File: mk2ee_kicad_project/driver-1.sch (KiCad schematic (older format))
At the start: 37 parts, among them J3 Conn_01x02_Male, J4 Conn_02x03_Male, J5 Conn_02x03_Male, J6 Conn_01x04_Male, J7 Conn_01x04_Male, U4 TSR_1-2465, U5 NCP718xSN330, U6 74HC595, U7 DRV8818PWP

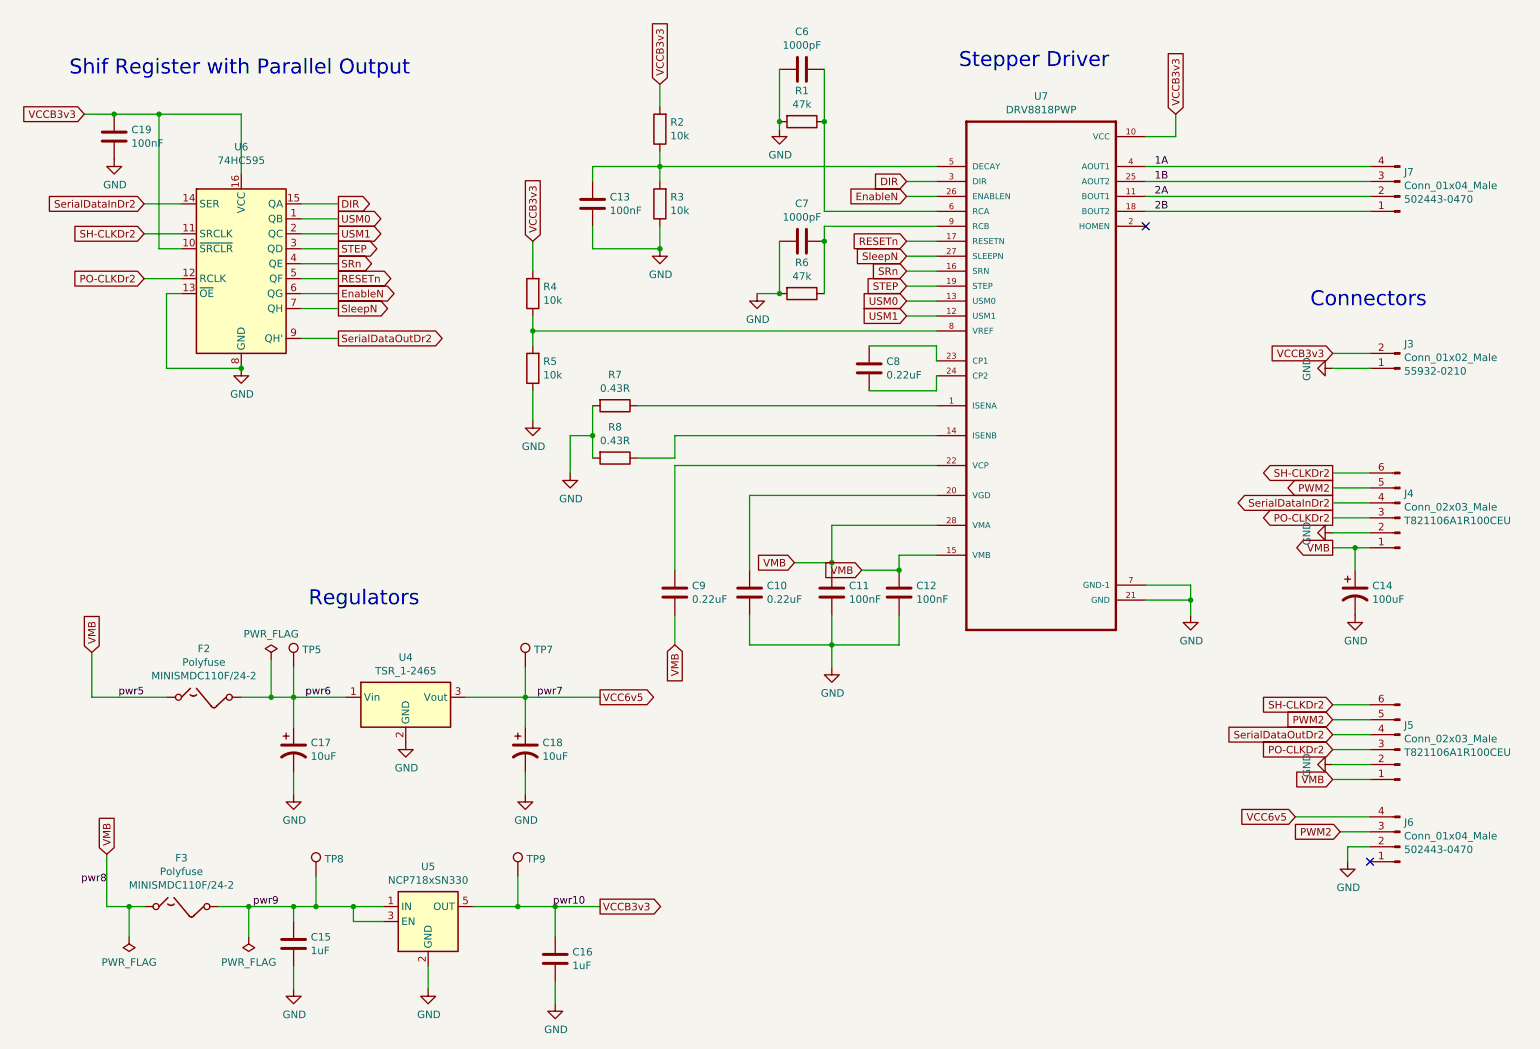
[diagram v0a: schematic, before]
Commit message: all components are connected
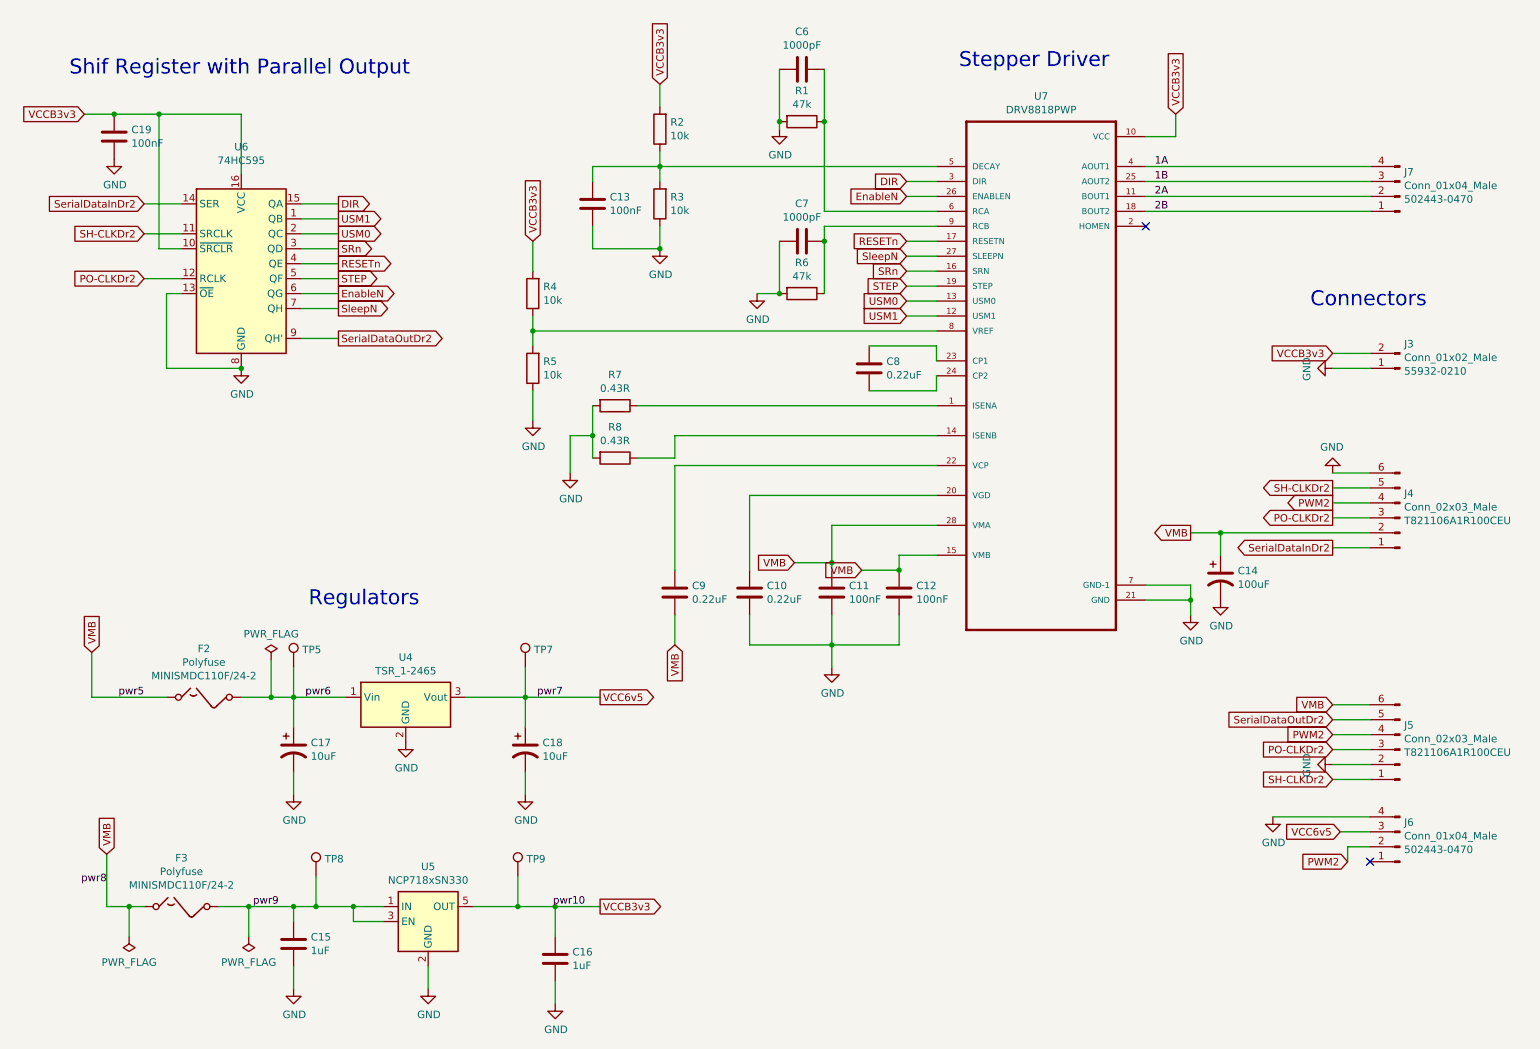
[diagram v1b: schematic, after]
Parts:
- TP5, TP7, TP8, TP9: footprint TestPoint:TestPoint_Pad_D4.0mm -> TestPoint:TestPoint_Pad_D1.5mm
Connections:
- net GND: now also J4.6 (Pin_6), J6.4 (Pin_4); no longer J4.2 (Pin_2), J6.2 (Pin_2)
- net PWM2: now also J4.4 (Pin_4), J5.4 (Pin_4), J6.2 (Pin_2); no longer J4.5 (Pin_5), J5.5 (Pin_5), J6.3 (Pin_3)
- net RESETn: now also U6.4 (QE); no longer U6.5 (QF)
- net SH-CLKDr2: now also J4.5 (Pin_5), J5.1 (Pin_1); no longer J4.6 (Pin_6), J5.6 (Pin_6)
- net SRn: now also U6.3 (QD); no longer U6.4 (QE)
- net STEP: now also U6.5 (QF); no longer U6.3 (QD)
- net SerialDataInDr2: now also J4.1 (Pin_1); no longer J4.4 (Pin_4)
- net SerialDataOutDr2: now also J5.5 (Pin_5); no longer J5.4 (Pin_4)
- net USM0: now also U6.2 (QC); no longer U6.1 (QB)
- net USM1: now also U6.1 (QB); no longer U6.2 (QC)
- net VCC6v5: now also J6.3 (Pin_3); no longer J6.4 (Pin_4)
- net VMB: now also J4.2 (Pin_2), J5.6 (Pin_6); no longer J4.1 (Pin_1), J5.1 (Pin_1)
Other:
- moved on the sheet: C14
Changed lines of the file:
@@
 L power:GND #PWR0117
 U 1 1 5F4EE14D
-P 9250 4050
-F 0 "#PWR0117" H 9250 3800 50  0001 C CNN
-F 1 "GND" H 9255 3877 50  0000 C CNN
-F 2 "" H 9250 4050 50  0001 C CNN
-F 3 "" H 9250 4050 50  0001 C CNN
-	1    9250 4050
-	0    1    1    0
-$EndComp
-Wire Wire Line
-	9250 4150 9400 4150
-Wire Wire Line
-	9250 4050 9500 4050
+P 9250 3650
+F 0 "#PWR0117" H 9250 3400 50  0001 C CNN
+F 1 "GND" H 9255 3477 50  0000 C CNN
+F 2 "" H 9250 3650 50  0001 C CNN
+F 3 "" H 9250 3650 50  0001 C CNN
+	1    9250 3650
+	-1   0    0    1
+$EndComp
 Text GLabel 2600 1850 2    50   Output ~ 0
 DIR
+Text GLabel 2600 2050 2    50   Output ~ 0
+USM0
 Text GLabel 2600 1950 2    50   Output ~ 0
-USM0
-Text GLabel 2600 2050 2    50   Output ~ 0
 USM1
+Text GLabel 2600 2350 2    50   Output ~ 0
+STEP
 Text GLabel 2600 2150 2    50   Output ~ 0
-STEP
+SRn
 Text GLabel 2600 2250 2    50   Output ~ 0
-SRn
-Text GLabel 2600 2350 2    50   Output ~ 0
 RESETn
+Text GLabel 9250 5300 0    50   Input ~ 0
+SerialDataOutDr2
 Text GLabel 9250 5400 0    50   Input ~ 0
-SerialDataOutDr2
-Text GLabel 9250 5300 0    50   Input ~ 0
 PWM2
-Text GLabel 9250 5200 0    50   Input ~ 0
+Text GLabel 9250 5700 0    50   Input ~ 0
 SH-CLKDr2
 Text GLabel 9250 5500 0    50   Input ~ 0
@@
 Text GLabel 1300 1850 0    50   Input ~ 0
 SerialDataInDr2
-Text GLabel 9250 5700 0    50   Input ~ 0
+Text GLabel 9250 5200 0    50   Input ~ 0
 VMB
 $Comp
@@
 Text GLabel 9250 3950 0    50   Output ~ 0
 PO-CLKDr2
-Text GLabel 9250 3650 0    50   Output ~ 0
+Text GLabel 9250 3750 0    50   Output ~ 0
 SH-CLKDr2
-Text GLabel 9250 3750 0    50   Output ~ 0
+Text GLabel 9250 3850 0    50   Output ~ 0
 PWM2
-Text GLabel 9250 3850 0    50   Output ~ 0
+Text GLabel 9250 4150 0    50   Output ~ 0
 SerialDataInDr2
 $Comp
@@
 Wire Wire Line
 	9250 2950 9500 2950
-Text GLabel 9250 4150 0    50   Output ~ 0
+Text GLabel 8300 4050 0    50   Output ~ 0
 VMB
-Wire Wire Line
-	9400 4300 9400 4150
-Connection ~ 9400 4150
-Wire Wire Line
-	9400 4150 9500 4150
 $Comp
 L power:GND #PWR0137
 U 1 1 5F975427
-P 9400 4600
-F 0 "#PWR0137" H 9400 4350 50  0001 C CNN
-F 1 "GND" H 9405 4427 50  0000 C CNN
-F 2 "" H 9400 4600 50  0001 C CNN
-F 3 "" H 9400 4600 50  0001 C CNN
-	1    9400 4600
+P 8500 4500
+F 0 "#PWR0137" H 8500 4250 50  0001 C CNN
+F 1 "GND" H 8505 4327 50  0000 C CNN
+F 2 "" H 8500 4500 50  0001 C CNN
+F 3 "" H 8500 4500 50  0001 C CNN
+	1    8500 4500
 	1    0    0    -1
 $EndComp
@@
 L power:GND #PWR0145
 U 1 1 5FC7793A
-P 9350 6250
-F 0 "#PWR0145" H 9350 6000 50  0001 C CNN
-F 1 "GND" H 9355 6077 50  0000 C CNN
-F 2 "" H 9350 6250 50  0001 C CNN
-F 3 "" H 9350 6250 50  0001 C CNN
-	1    9350 6250
-	1    0    0    -1
-$EndComp
-Text GLabel 9000 5950 0    50   Input ~ 0
+P 8850 5950
+F 0 "#PWR0145" H 8850 5700 50  0001 C CNN
+F 1 "GND" H 8855 5777 50  0000 C CNN
+F 2 "" H 8850 5950 50  0001 C CNN
+F 3 "" H 8850 5950 50  0001 C CNN
+	1    8850 5950
+	1    0    0    -1
+$EndComp
+Text GLabel 9300 6050 0    50   Input ~ 0
 VCC6v5
 Wire Wire Line
-	9000 5950 9500 5950
-Wire Wire Line
 	9350 6250 9350 6150
 Wire Wire Line
 	9350 6150 9500 6150
-Text GLabel 9300 6050 0    50   Input ~ 0
+Text GLabel 9350 6250 0    50   Input ~ 0
 PWM2
 Wire Wire Line
@@
 L Device:CP1 C?
 U 1 1 602E4B0B
-P 9400 4450
+P 8500 4350
 AR Path="/5F455032/602E4B0B" Ref="C?"  Part="1"
 AR Path="/5F4C637B/602E4B0B" Ref="C?"  Part="1"
 AR Path="/5F475AB3/602E4B0B" Ref="C14"  Part="1"
-F 0 "C14" H 9515 4496 50  0000 L CNN
-F 1 "100uF" H 9515 4405 50  0000 L CNN
-F 2 "Capacitor_SMD:CP_Elec_6.3x7.7" H 9400 4450 50  0001 C CNN
-F 3 "~" H 9400 4450 50  0001 C CNN
-F 4 "EEEFK1E101XP" H 9400 4450 50  0001 C CNN "Name"
-F 5 "Panasonic" H 9400 4450 50  0001 C CNN "Manufacturer"
-	1    9400 4450
+F 0 "C14" H 8615 4396 50  0000 L CNN
+F 1 "100uF" H 8615 4305 50  0000 L CNN
+F 2 "Capacitor_SMD:CP_Elec_6.3x7.7" H 8500 4350 50  0001 C CNN
+F 3 "~" H 8500 4350 50  0001 C CNN
+F 4 "EEEFK1E101XP" H 8500 4350 50  0001 C CNN "Name"
+F 5 "Panasonic" H 8500 4350 50  0001 C CNN "Manufacturer"
+	1    8500 4350
 	1    0    0    -1
 $EndComp
@@
 F 0 "TP5" H 2358 5068 50  0000 L CNN
 F 1 "TestPoint" H 2358 4977 50  0001 L CNN
-F 2 "TestPoint:TestPoint_Pad_D4.0mm" H 2500 4950 50  0001 C CNN
+F 2 "TestPoint:TestPoint_Pad_D1.5mm" H 2500 4950 50  0001 C CNN
 F 3 "~" H 2500 4950 50  0001 C CNN
 	1    2300 4950
@@
 F 0 "TP7" H 3908 5068 50  0000 L CNN
 F 1 "TestPoint" H 3908 4977 50  0001 L CNN
-F 2 "TestPoint:TestPoint_Pad_D4.0mm" H 4050 4950 50  0001 C CNN
+F 2 "TestPoint:TestPoint_Pad_D1.5mm" H 4050 4950 50  0001 C CNN
 F 3 "~" H 4050 4950 50  0001 C CNN
 	1    3850 4950
@@
 F 0 "TP8" H 2508 6468 50  0000 L CNN
 F 1 "TestPoint" H 2508 6377 50  0001 L CNN
-F 2 "TestPoint:TestPoint_Pad_D4.0mm" H 2650 6350 50  0001 C CNN
+F 2 "TestPoint:TestPoint_Pad_D1.5mm" H 2650 6350 50  0001 C CNN
 F 3 "~" H 2650 6350 50  0001 C CNN
 	1    2450 6350
@@
 F 0 "TP9" H 3858 6468 50  0000 L CNN
 F 1 "TestPoint" H 3858 6377 50  0001 L CNN
-F 2 "TestPoint:TestPoint_Pad_D4.0mm" H 4000 6350 50  0001 C CNN
+F 2 "TestPoint:TestPoint_Pad_D1.5mm" H 4000 6350 50  0001 C CNN
 F 3 "~" H 4000 6350 50  0001 C CNN
 	1    3800 6350
@@
 Wire Wire Line
 	5850 2100 5850 2450
+Wire Wire Line
+	8850 5950 9500 5950
+Wire Wire Line
+	9250 4150 9500 4150
+Wire Wire Line
+	8300 4050 8500 4050
+Wire Wire Line
+	8500 4200 8500 4050
+Connection ~ 8500 4050
+Wire Wire Line
+	8500 4050 9500 4050
 $EndSCHEMATC
